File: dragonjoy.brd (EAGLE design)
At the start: 67.3 x 49.5 mm, 24 parts, among them IC1 4066N, IC2 4066N

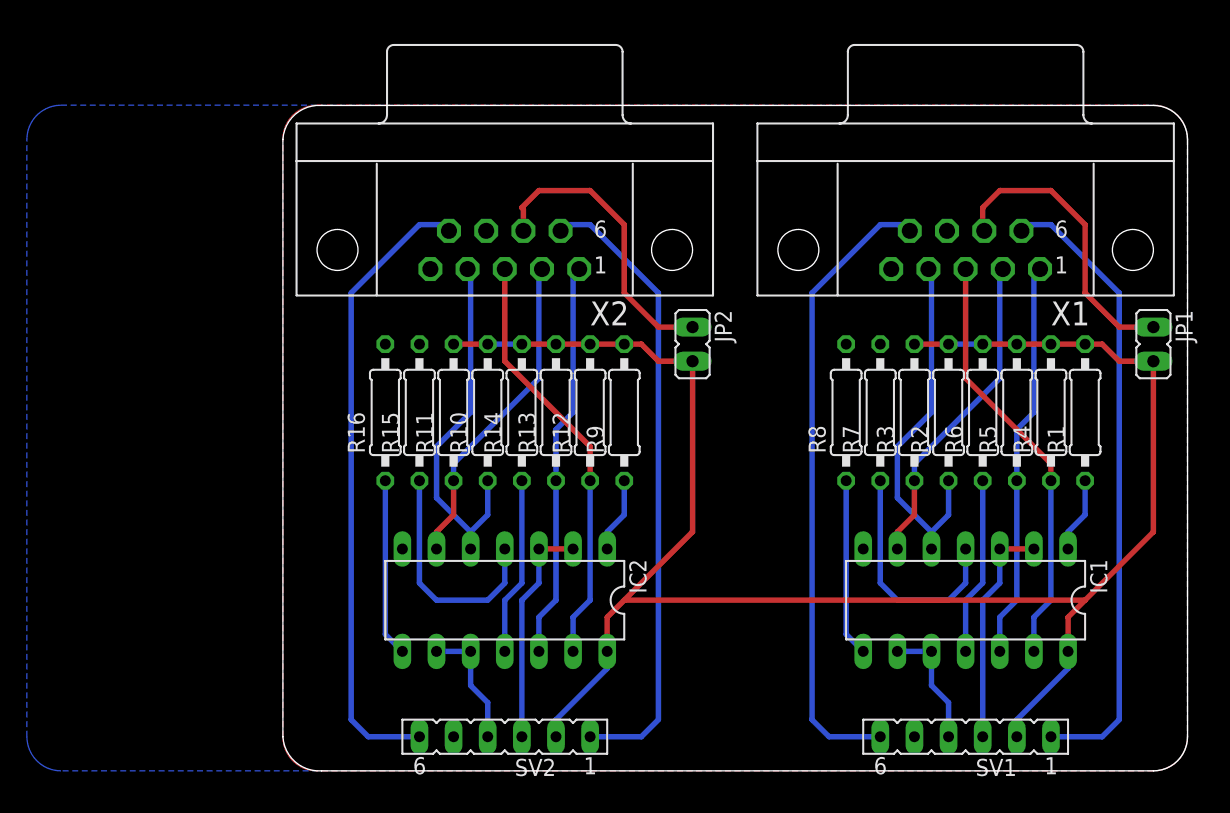
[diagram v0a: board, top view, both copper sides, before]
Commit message: prepare for submission
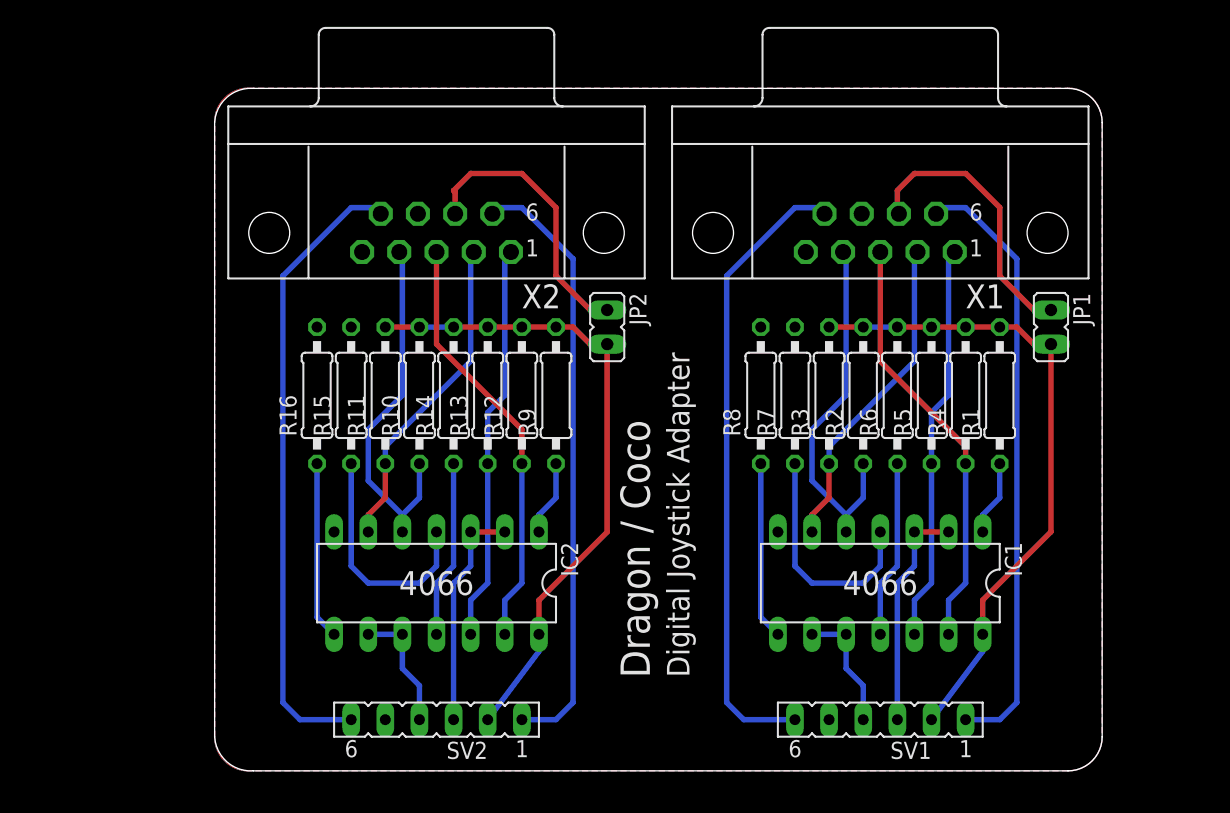
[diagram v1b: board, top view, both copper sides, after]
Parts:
- moved JP1 7.73 mm to (29.2, 33.0)
- moved R1 6.48 mm to (25.4, 27.9)
- moved R3 6.48 mm to (12.7, 27.9)
- moved R4 6.48 mm to (22.9, 27.9)
- moved R5 6.48 mm to (20.3, 27.9)
- moved R7 6.48 mm to (10.2, 27.9)
- moved R8 6.48 mm to (7.62, 27.9)
- moved JP2 6.48 mm to (-3.81, 33.0)
- moved R2 6.48 mm to (15.2, 27.9)
- moved IC1 6.48 mm to (16.5, 14.0)
- moved R6 6.48 mm to (17.8, 27.9)
- moved SV1 6.48 mm to (16.5, 3.81)
- moved X1 6.48 mm to (16.5, 49.5)
- moved IC2 5.24 mm to (-16.5, 14.0)
- moved R10 5.24 mm to (-17.8, 27.9)
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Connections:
- net N$7 renamed N$7-R
- new net VCC-R: IC2.14, JP2.2, R10.2, R11.2, R12.2, R13.2, R14.2, R9.2, SV2.2
- net VCC: no longer IC2.14, JP2.2, R10.2, R11.2, R12.2, R13.2, R14.2, R9.2, SV2.2
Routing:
- net VCC: track 135.2 -> 48.4 mm
- net VCC-R: track 0.00 -> 48.4 mm
- net FIRE-R: track 46.9 -> 45.1 mm
- net FIRE: track 46.9 -> 45.1 mm
- net N$7-R: track 22.2 -> 20.9 mm
- net N$1: track 22.2 -> 20.9 mm
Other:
- board size 67.3 x 49.5 mm -> 66 x 50.8 mm
- board text added: "4066"
- board text added: "Digital Joystick Adapter"
- board text added: "Dragon / Coco"
